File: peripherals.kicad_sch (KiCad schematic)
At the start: 21 parts, among them J12 0533980471, J13 QSH-030-01-L-D-A, J14 QTH-030-01-L-D-A, U23 NTS0102, U24 NTS0102, U25 NTS0102, U26 MAX3051

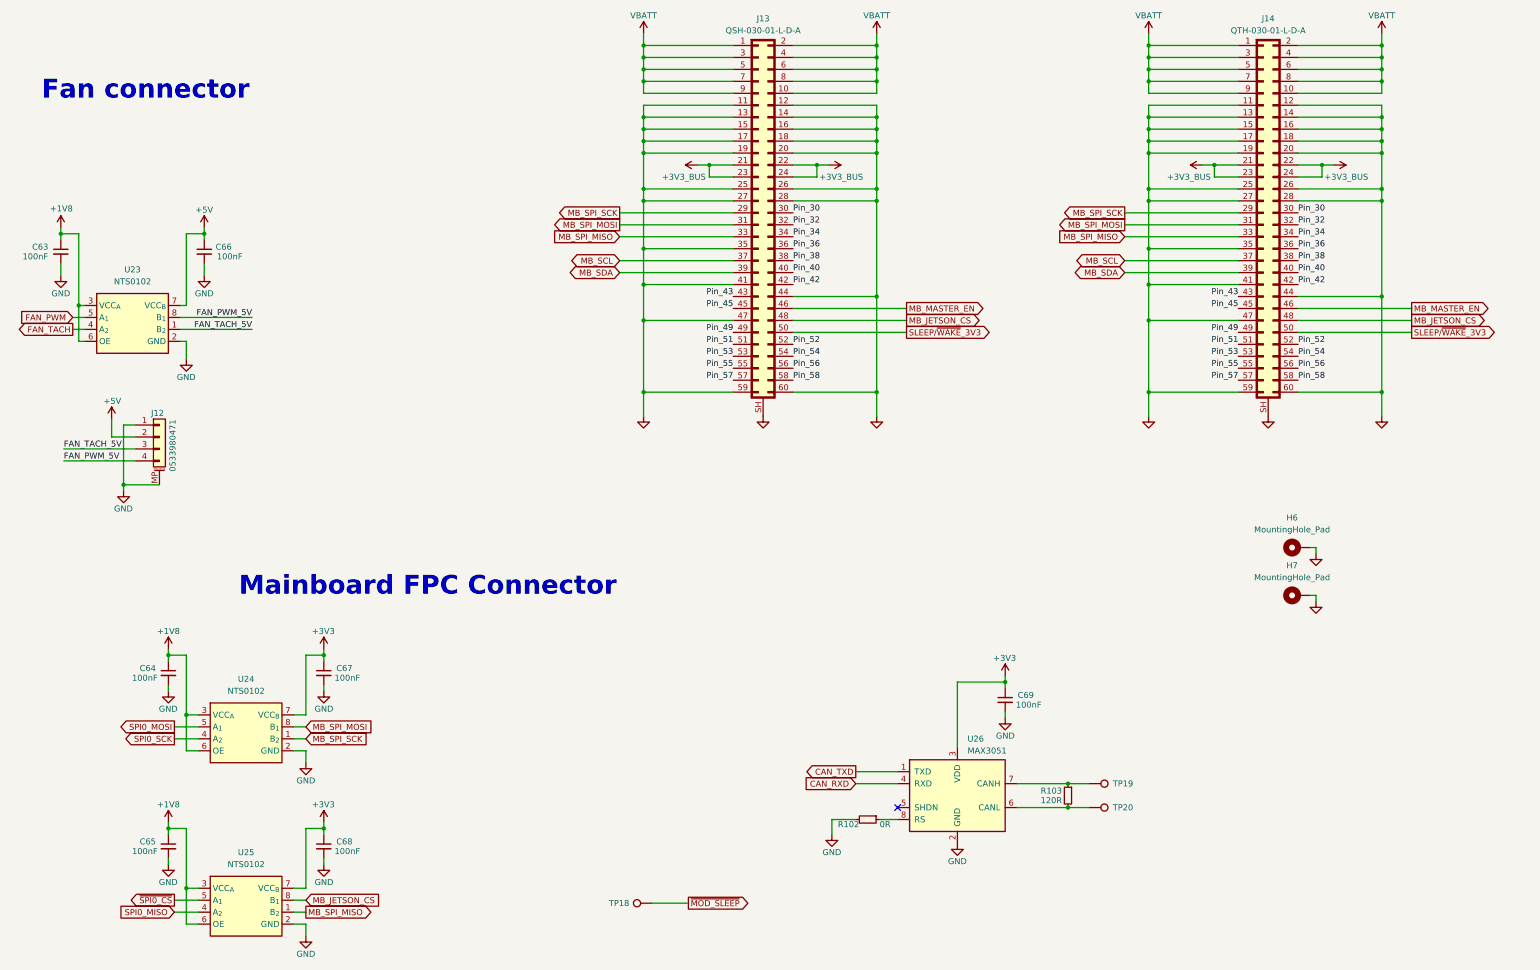
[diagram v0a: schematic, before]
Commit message: Final BOM changes, gerbers
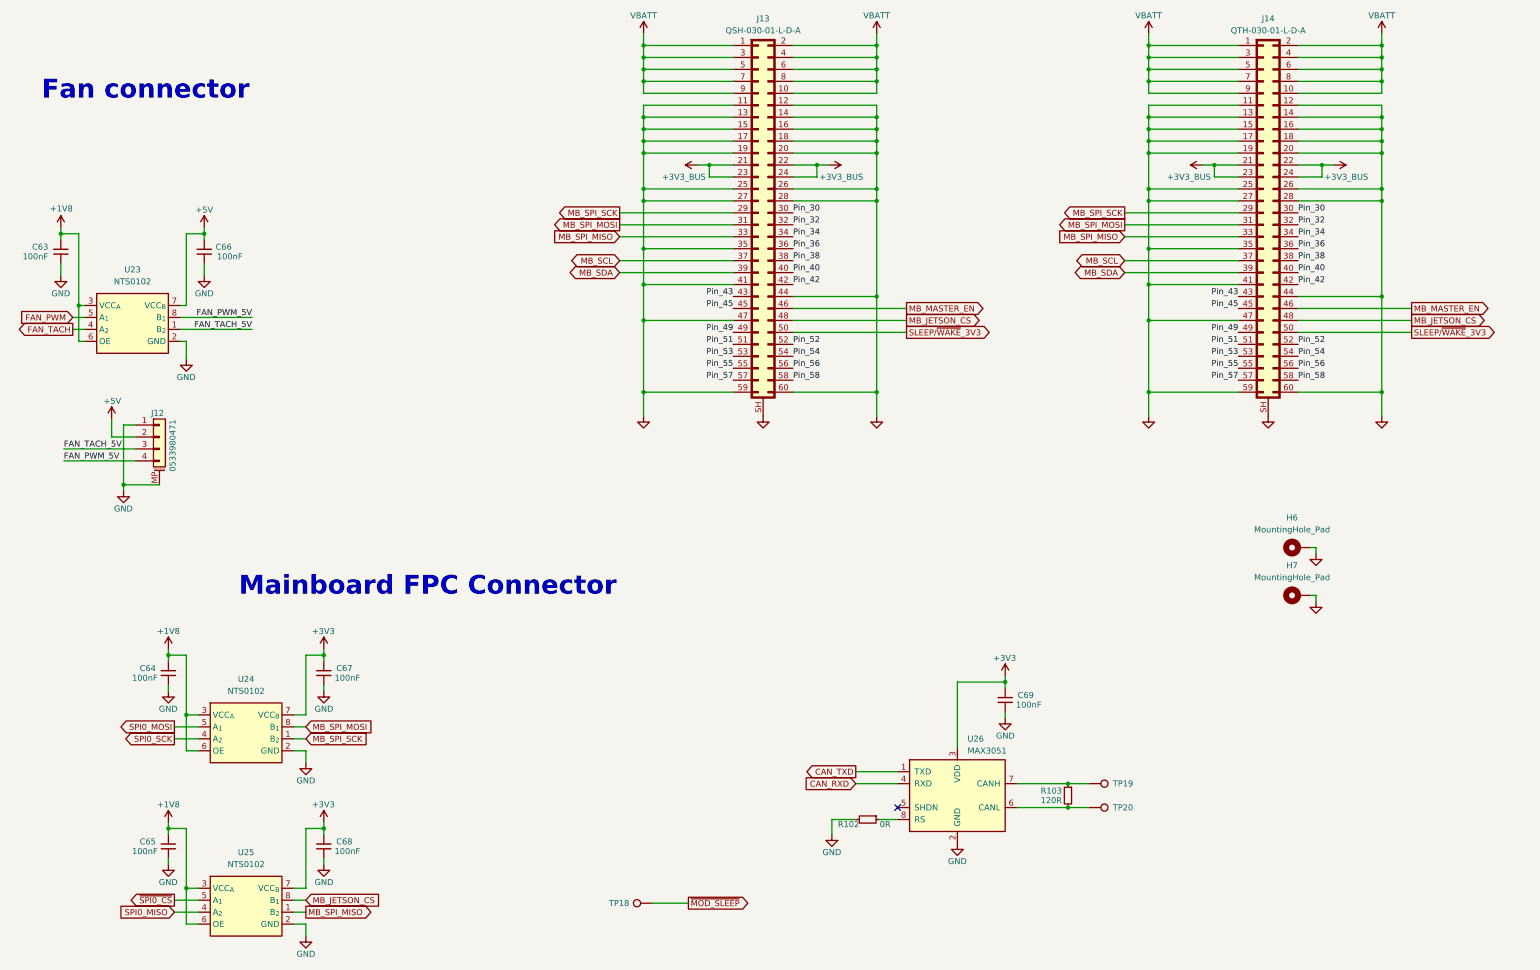
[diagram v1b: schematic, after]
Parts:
- C63, C64, C65, C66, C67, C68, C69: LCSC (none) -> C14663
- J12: LCSC (none) -> C17617036
- J13: LCSC (none) -> C2909821
- J14: LCSC (none) -> C2843756
- R102: LCSC (none) -> C21189
- R103: LCSC (none) -> C22787
- U23, U24, U25: LCSC (none) -> C2687851
- U26: LCSC (none) -> C112005
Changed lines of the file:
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@@
 			)
 		)
+		(property "LCSC" "C22787"
+			(at 254.635 237.109 0)
+			(effects
+				(font
+					(size 1.27 1.27)
+				)
+				(hide yes)
+			)
+		)
 		(pin "2"
 		)
@@
 			)
 		)
+		(property "LCSC" "C2687851"
+			(at 57.15 126.365 0)
+			(effects
+				(font
+					(size 1.27 1.27)
+				)
+				(hide yes)
+			)
+		)
 		(pin "4"
 		)
@@
 			)
 		)
+		(property "LCSC" "C2687851"
+			(at 81.28 213.36 0)
+			(effects
+				(font
+					(size 1.27 1.27)
+				)
+				(hide yes)
+			)
+		)
 		(pin "4"
 		)
@@
 			)
 		)
+		(property "LCSC" "C21189"
+			(at 207.01 244.983 0)
+			(effects
+				(font
+					(size 1.27 1.27)
+				)
+				(hide yes)
+			)
+		)
 		(pin "1"
 		)
@@
 			)
 		)
+		(property "LCSC" "C2843756"
+			(at 298.45 73.025 0)
+			(effects
+				(font
+					(size 1.27 1.27)
+				)
+				(hide yes)
+			)
+		)
 		(pin "19"
 		)
@@
 			)
 		)
+		(property "LCSC" "C14663"
+			(at 103.886 211.074 0)
+			(effects
+				(font
+					(size 1.27 1.27)
+				)
+				(hide yes)
+			)
+		)
 		(pin "1"
 		)
@@
 			)
 		)
+		(property "LCSC" "C112005"
+			(at 234.5533 226.06 0)
+			(effects
+				(font
+					(size 1.27 1.27)
+				)
+				(hide yes)
+			)
+		)
 		(pin "2"
 		)
@@
 			)
 		)
+		(property "LCSC" "C14663"
+			(at 103.886 247.904 0)
+			(effects
+				(font
+					(size 1.27 1.27)
+				)
+				(hide yes)
+			)
+		)
 		(pin "1"
 		)
@@
 			)
 		)
+		(property "LCSC" "C14663"
+			(at 35.814 121.539 0)
+			(effects
+				(font
+					(size 1.27 1.27)
+				)
+				(hide yes)
+			)
+		)
 		(pin "1"
 		)
@@
 			)
 		)
+		(property "LCSC" "C14663"
+			(at 58.674 211.074 0)
+			(effects
+				(font
+					(size 1.27 1.27)
+				)
+				(hide yes)
+			)
+		)
 		(pin "1"
 		)
@@
 			)
 		)
+		(property "LCSC" "C14663"
+			(at 58.674 247.904 0)
+			(effects
+				(font
+					(size 1.27 1.27)
+				)
+				(hide yes)
+			)
+		)
 		(pin "1"
 		)
@@
 			)
 		)
+		(property "LCSC" "C14663"
+			(at 78.232 121.539 0)
+			(effects
+				(font
+					(size 1.27 1.27)
+				)
+				(hide yes)
+			)
+		)
 		(pin "1"
 		)
@@
 			)
 		)
+		(property "LCSC" "C14663"
+			(at 248.666 216.789 0)
+			(effects
+				(font
+					(size 1.27 1.27)
+				)
+				(hide yes)
+			)
+		)
 		(pin "1"
 		)
@@
 			)
 		)
+		(property "LCSC" "C17617036"
+			(at 61.087 156.845 0)
+			(effects
+				(font
+					(size 1.27 1.27)
+				)
+				(hide yes)
+			)
+		)
 		(pin "1"
 		)
@@
 			)
 		)
+		(property "LCSC" "C2687851"
+			(at 81.28 250.19 0)
+			(effects
+				(font
+					(size 1.27 1.27)
+				)
+				(hide yes)
+			)
+		)
 		(pin "4"
 		)
@@
 			)
 		)
+		(property "LCSC" "C2909821"
+			(at 191.135 73.025 0)
+			(effects
+				(font
+					(size 1.27 1.27)
+				)
+				(hide yes)
+			)
+		)
